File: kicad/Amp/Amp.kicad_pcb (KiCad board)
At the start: 2 copper layers, 30 x 25.6 mm, 31 parts, among them J1 Conn, J2 Conn, J3 Conn, J4 Conn, J5 Conn, U1 TS5A3166DBVR, U2 MCP1700

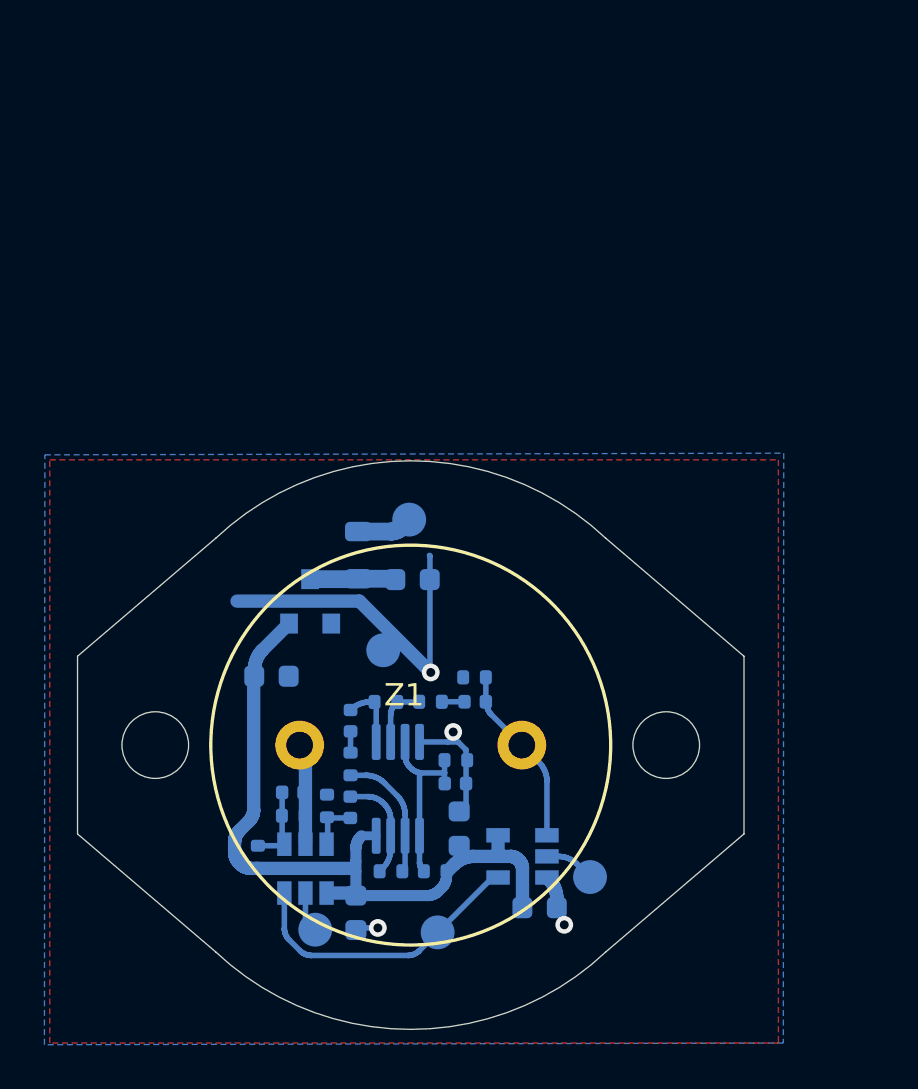
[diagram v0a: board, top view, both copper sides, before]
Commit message: изменено:      kicad/Amp/Amp.kicad_pcb 	изменено:      kicad/Amp/Amp.kicad_pcb-bak 	изменено:      kicad/Amp/Amp.sch 	изменено:      kicad/Amp/Amp.sch-bak 	изменено:      stm32cubeide/Anemometr_v3/.mxproject 	изменено:      stm32cubeide/Anemometr_v3/Anemometr_3.ioc 	изменено:      stm32cubeide/Anemometr_v3/Core/Inc/main.h 	изменено:      stm32cubeide/Anemometr_v3/Core/Inc/stm32f1xx_hal_conf.h 	изменено:      stm32cubeide/Anemometr_v3/Core/Src/main.c 	изменено:      stm32cubeide/Anemometr_v3/Core/Src/stm32f1xx_it.c 	изменено:      stm32cubeide/Anemometr_v3/Debug/Anemometr_3.bin 	изменено:      stm32cubeide/Anemometr_v3/Debug/Anemometr_3.elf 	изменено:      stm32cubeide/Anemometr_v3/Debug/Anemometr_3.list 	изменено:      stm32cubeide/Anemometr_v3/Debug/Anemometr_3.map 	изменено:      stm32cubeide/Anemometr_v3/Debug/Core/Src/BME280.d 	изменено:      stm32cubeide/Anemometr_v3/Debug/Core/Src/BME280.o 	изменено:      stm32cubeide/Anemometr_v3/Debug/Core/Src/main.d 	изменено:      stm32cubeide/Anemometr_v3/Debug/Core/Src/main.o 	изменено:      stm32cubeide/Anemometr_v3/Debug/Core/Src/main.su 	изменено:      stm32cubeide/Anemometr_v3/Debug/Core/Src/stm32f1xx_hal_msp.d 	изменено:      stm32cubeide/Anemometr_v3/Debug/Core/Src/stm32f1xx_hal_msp.o 	изменено:      stm32cubeide/Anemometr_v3/Debug/Core/Src/stm32f1xx_it.d 	изменено:      stm32cubeide/Anemometr_v3/Debug/Core/Src/stm32f1xx_it.o 	изменено:      stm32cubeide/Anemometr_v3/Debug/Core/Src/stm32f1xx_it.su 	изменено:      stm32cubeide/Anemometr_v3/Debug/Core/Src/system_stm32f1xx.d 	изменено:      stm32cubeide/Anemometr_v3/Debug/Core/Src/system_stm32f1xx.o 	изменено:      stm32cubeide/Anemometr_v3/Debug/Drivers/STM32F1xx_HAL_Driver/Src/stm32f1xx_hal.d 	изменено:      stm32cubeide/Anemometr_v3/Debug/Drivers/STM32F1xx_HAL_Driver/Src/stm32f1xx_hal.o 	изменено:      stm32cubeide/Anemometr_v3/Debug/Drivers/STM32F1xx_HAL_Driver/Src/stm32f1xx_hal_cortex.d 	изменено:      stm32cubeide/Anemometr_v3/Debug/Drivers/STM32F1xx_HAL_Driver/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
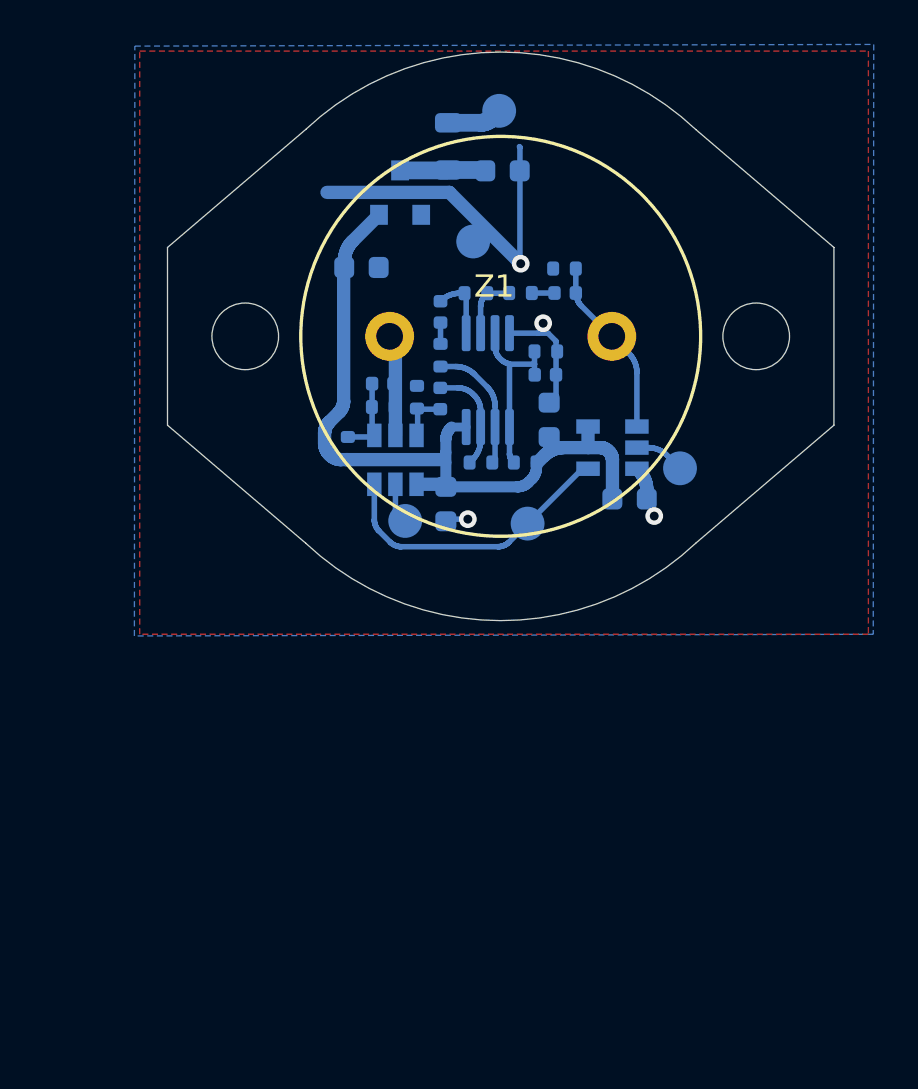
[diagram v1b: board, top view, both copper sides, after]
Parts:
- R5: value 100k -> 390k
- moved C4 18.8 mm to (44.3, 58.2)
- moved C5 18.8 mm to (40.8, 56.2)
- moved C8 18.8 mm to (52.9, 66.6)
- moved D2 18.8 mm to (42.3, 64.8)
- moved R6 18.8 mm to (44.3, 60.1)
- moved R8 18.8 mm to (43.3, 62.0)
- moved R9 18.8 mm to (40.2, 64.3)
- moved C9 18.8 mm to (49.2, 63.0)
- moved J2 18.8 mm to (42.8, 67.6)
- moved J4 18.8 mm to (48.3, 67.7)
- moved J5 18.8 mm to (47.0, 49.1)
- moved R10 18.8 mm to (41.8, 62.5)
- moved R3 18.8 mm to (48.1, 65.0)
- moved R4 18.8 mm to (49.1, 60.0)
- moved R7 18.8 mm to (46.2, 65.0)
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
